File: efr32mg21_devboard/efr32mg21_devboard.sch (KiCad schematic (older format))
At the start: 23 parts, among them CON1 CORTEX-DEBUGGER, J1 Conn_01x10, J2 microusb, U1 EFR32MG21A020F768IM32-BR, U2 TLV70033_SOT23-5, Y1 38.4MHz, Y2 32.768k

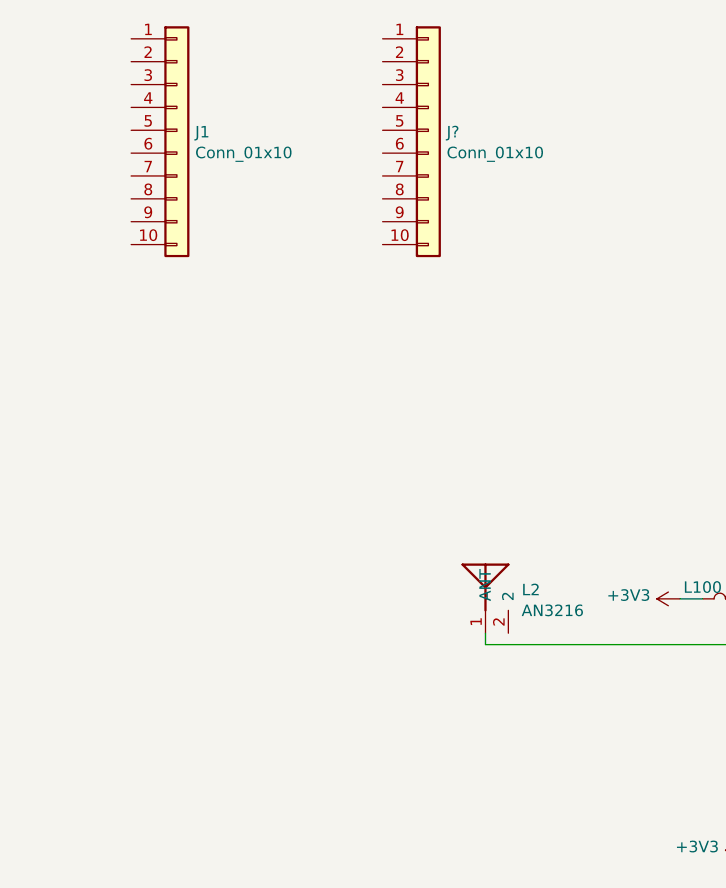
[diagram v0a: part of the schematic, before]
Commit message: pcb
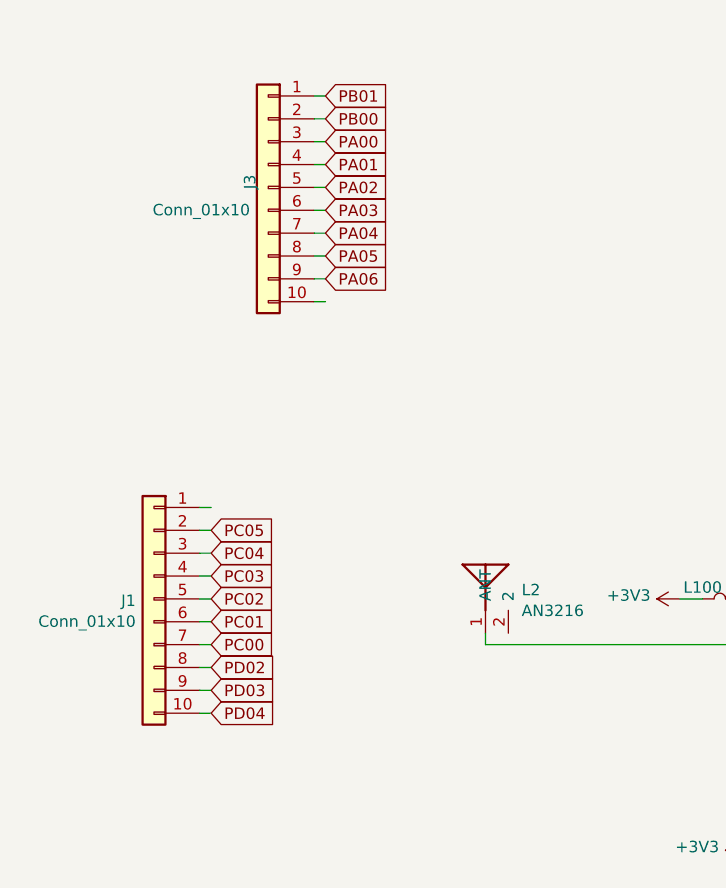
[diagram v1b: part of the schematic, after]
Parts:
- gave numbers to parts that had none: 1
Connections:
- wire segments 104 -> 124
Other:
- moved on the sheet: J1, J3
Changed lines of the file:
@@
 L Connector_Generic:Conn_01x10 J1
 U 1 1 60A40A6A
-P 1400 1450
-F 0 "J1" H 1480 1442 50  0000 L CNN
-F 1 "Conn_01x10" H 1480 1351 50  0000 L CNN
-F 2 "Connector_PinHeader_2.54mm:PinHeader_1x10_P2.54mm_Vertical" H 1400 1450 50  0001 C CNN
-F 3 "~" H 1400 1450 50  0001 C CNN
-	1    1400 1450
-	1    0    0    -1
+P 1300 3500
+F 0 "J1" H 1380 3492 50  0000 L CNN
+F 1 "Conn_01x10" H 1380 3401 50  0000 L CNN
+F 2 "Connector_PinHeader_2.54mm:PinHeader_1x10_P2.54mm_Vertical" H 1300 3500 50  0001 C CNN
+F 3 "~" H 1300 3500 50  0001 C CNN
+	1    1300 3500
+	-1   0    0    -1
 $EndComp
 $Comp
@@
 $EndComp
 $Comp
-L Connector_Generic:Conn_01x10 J?
+L Connector_Generic:Conn_01x10 J3
 U 1 1 60A33E9A
-P 2500 1450
-F 0 "J?" H 2580 1442 50  0000 L CNN
-F 1 "Conn_01x10" H 2580 1351 50  0000 L CNN
-F 2 "Connector_PinHeader_2.54mm:PinHeader_1x10_P2.54mm_Vertical" H 2500 1450 50  0001 C CNN
-F 3 "~" H 2500 1450 50  0001 C CNN
-	1    2500 1450
-	1    0    0    -1
+P 1800 1700
+F 0 "J3" V 1880 1692 50  0000 L CNN
+F 1 "Conn_01x10" H 1880 1601 50  0000 L CNN
+F 2 "Connector_PinHeader_2.54mm:PinHeader_1x10_P2.54mm_Vertical" H 1800 1700 50  0001 C CNN
+F 3 "~" H 1800 1700 50  0001 C CNN
+	1    1800 1700
+	-1   0    0    -1
 $EndComp
+Wire Wire Line
+	2050 1300 2000 1300
+Wire Wire Line
+	2050 1400 2000 1400
+Wire Wire Line
+	2050 1500 2000 1500
+Wire Wire Line
+	2050 1600 2000 1600
+Wire Wire Line
+	2050 1700 2000 1700
+Wire Wire Line
+	2050 1800 2000 1800
+Wire Wire Line
+	2050 1900 2000 1900
+Wire Wire Line
+	2050 2000 2000 2000
+Wire Wire Line
+	2050 2100 2000 2100
+Wire Wire Line
+	2050 2200 2000 2200
+Text GLabel 2050 1300 2    50   Input ~ 0
+PB01
+Text GLabel 2050 1400 2    50   Input ~ 0
+PB00
+Text GLabel 2050 1500 2    50   Input ~ 0
+PA00
+Text GLabel 2050 1600 2    50   Input ~ 0
+PA01
+Text GLabel 2050 1700 2    50   Input ~ 0
+PA02
+Text GLabel 2050 1800 2    50   Input ~ 0
+PA03
+Text GLabel 2050 1900 2    50   Input ~ 0
+PA04
+Text GLabel 2050 2000 2    50   Input ~ 0
+PA05
+Text GLabel 2050 2100 2    50   Input ~ 0
+PA06
+Wire Wire Line
+	1550 4000 1500 4000
+Wire Wire Line
+	1550 3900 1500 3900
+Wire Wire Line
+	1550 3800 1500 3800
+Wire Wire Line
+	1550 3700 1500 3700
+Wire Wire Line
+	1550 3600 1500 3600
+Wire Wire Line
+	1550 3500 1500 3500
+Wire Wire Line
+	1550 3400 1500 3400
+Wire Wire Line
+	1550 3300 1500 3300
+Wire Wire Line
+	1550 3200 1500 3200
+Wire Wire Line
+	1550 3100 1500 3100
+Text GLabel 1550 4000 2    50   Input ~ 0
+PD04
+Text GLabel 1550 3900 2    50   Input ~ 0
+PD03
+Text GLabel 1550 3800 2    50   Input ~ 0
+PD02
+Text GLabel 1550 3700 2    50   Input ~ 0
+PC00
+Text GLabel 1550 3600 2    50   Input ~ 0
+PC01
+Text GLabel 1550 3500 2    50   Input ~ 0
+PC02
+Text GLabel 1550 3400 2    50   Input ~ 0
+PC03
+Text GLabel 1550 3300 2    50   Input ~ 0
+PC04
+Text GLabel 1550 3200 2    50   Input ~ 0
+PC05
 $EndSCHEMATC
